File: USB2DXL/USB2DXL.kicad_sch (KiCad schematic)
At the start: 13 parts, among them J1 Conn_01x02, J2 USB_C_Receptacle_USB2.0_16P, U1 CH340E

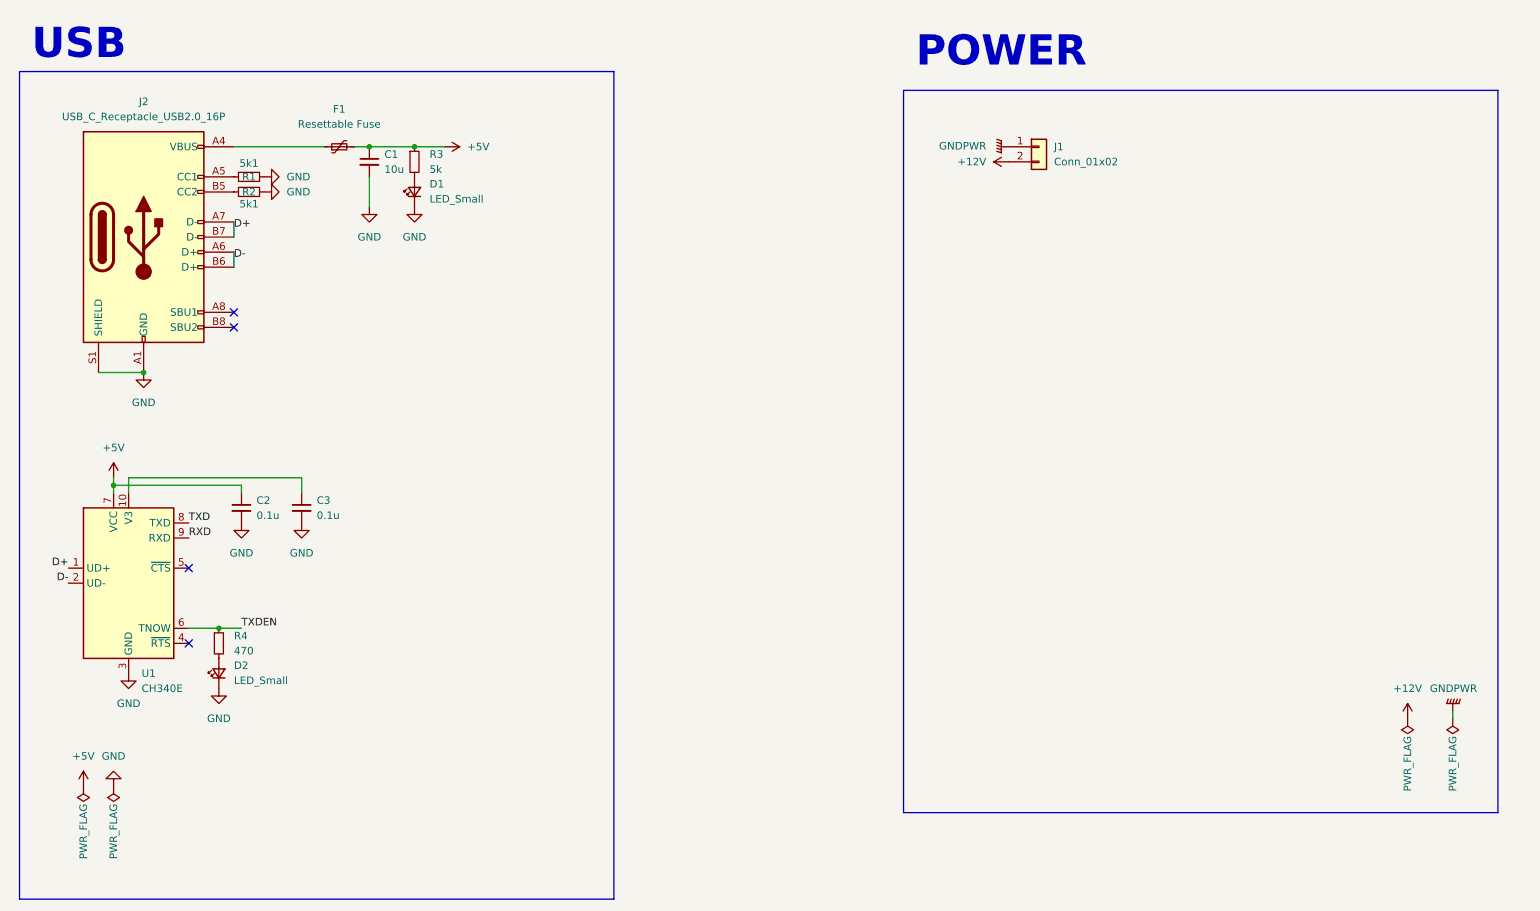
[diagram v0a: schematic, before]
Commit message: 仮
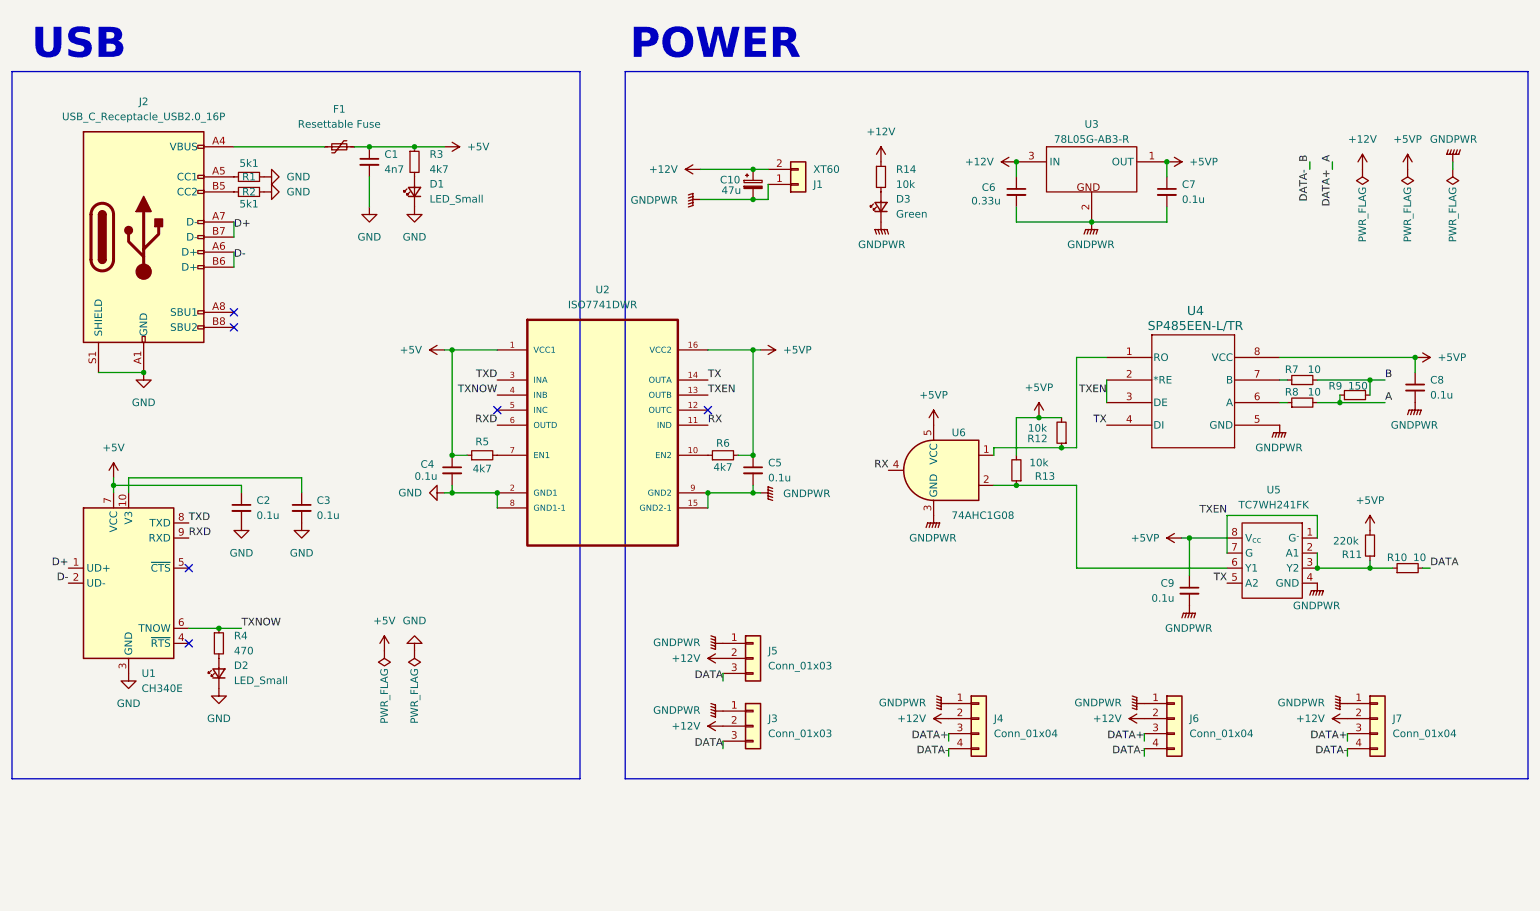
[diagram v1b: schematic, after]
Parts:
- added C10: 47u, Capacitor_THT:CP_Radial_D5.0mm_P2.00mm, symbol Device:C_Polarized_Small
- added C4, C5, C7, C8, C9: 0.1u, Capacitor_SMD:C_0402_1005Metric, symbol Device:C_Small
- added C6: 0.33u, Capacitor_SMD:C_0603_1608Metric, symbol Device:C_Small
- added D3: Green, LED_SMD:LED_0805_2012Metric_Pad1.15x1.40mm_HandSolder, symbol Device:LED_Small
- added J3, J5: Conn_01x03, Connector_JST:JST_EH_B3B-EH-A_1x03_P2.50mm_Vertical, symbol Connector_Generic:Conn_01x03
- added J4, J6, J7: Conn_01x04, Connector_Molex:Molex_SPOX_5267-04A_1x04_P2.50mm_Vertical, symbol Connector_Generic:Conn_01x04
- added R10, R7, R8: 10, Resistor_SMD:R_0402_1005Metric, symbol Device:R_Small
- added R11: 220k, Resistor_SMD:R_0402_1005Metric, symbol Device:R_Small
- added R12, R14: 10k, Resistor_SMD:R_0402_1005Metric, symbol Device:R_Small
- added R13: 10k, Capacitor_SMD:C_0402_1005Metric, symbol Device:R_Small
- added R5, R6: 4k7, Resistor_SMD:R_0402_1005Metric, symbol Device:R_Small
- added R9: 150, Resistor_SMD:R_0402_1005Metric, symbol Device:R_Small
- added U2: ISO7741DWR, ISO7741DWR:SOIC127P1030X265-16N, symbol ISO7741DWR:ISO7741DWR
- added U3: 78L05G-AB3-R, Package_TO_SOT_SMD:SOT-89-3, symbol ProLib_pcs_2025-07-07:78L05G-AB3-R
- added U4: SP485EEN-L/TR, SP485EEN-L/TR:NSOIC-8, symbol SP485EEN-L/TR:SP485EEN-L_TR
- added U5: TC7WH241FK, Package_SO:MSOP-8_3x3mm_P0.65mm, symbol MyLibrary:TC7WH241FK
- added U6: 74AHC1G08, Package_TO_SOT_SMD:SOT-23-5_HandSoldering, symbol 74xGxx:74AHC1G08
- C1: value 10u -> 4n7; footprint (none) -> Capacitor_SMD:C_0402_1005Metric
- C2, C3: footprint (none) -> Capacitor_SMD:C_0402_1005Metric
- D1, D2: footprint (none) -> LED_SMD:LED_0603_1608Metric
- J1: value Conn_01x02 -> XT60
- R1, R2, R4: footprint (none) -> Resistor_SMD:R_0402_1005Metric
- R3: value 5k -> 4k7; footprint (none) -> Resistor_SMD:R_0402_1005Metric
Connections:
- net +12V: now also C10.1, C6.1, J3.2 (Pin_2), J4.2 (Pin_2), J5.2 (Pin_2), J6.2 (Pin_2), J7.2 (Pin_2), R14.1, U3.3 (IN)
- net +5V: now also C4.1, R5.1, U2.1 (VCC1)
- net GND: now also C4.2, U2.2 (GND1), U2.8 (GND1-1)
- net GNDPWR: now also C10.2, C5.2, C6.2, C7.2, C8.2, C9.2, D3.1 (K), J3.1 (Pin_1), J4.1 (Pin_1), J5.1 (Pin_1), J6.1 (Pin_1), J7.1 (Pin_1), U2.15 (GND2-1), U2.9 (GND2), U3.2 (GND), U4.5 (GND), U5.4 (GND), U6.3 (GND)
- net RXD: now also U2.6 (OUTD)
- net TXD: now also U2.3 (INA)
- net TXDEN renamed TXNOW
- net TXNOW: now also U2.4 (INB)
- new net: R13.1, U5.6 (Y1), U6.2
- new net: R12.1, U4.1 (RO), U6.1
- new net: R8.1, U4.6 (A)
- new net: R7.1, U4.7 (B)
- new net: R10.1, R11.1, U5.2 (A1), U5.3 (Y2)
- new net: R5.2, U2.7 (EN1)
- new net: D3.2 (A), R14.2
- new net: R6.1, U2.10 (EN2)
- new net +5VP: C5.1, C7.1, C8.1, C9.1, R11.2, R12.2, R13.2, R6.2, U2.16 (VCC2), U3.1 (OUT), U4.8 (VCC), U5.8 (V_{cc}), U6.5 (VCC)
- new net A: J4.3 (Pin_3), J6.3 (Pin_3), J7.3 (Pin_3), R8.2, R9.1
- new net B: J4.4 (Pin_4), J6.4 (Pin_4), J7.4 (Pin_4), R7.2, R9.2
- new net DATA: J3.3 (Pin_3), J5.3 (Pin_3), R10.2
- new net RX: U2.11 (IND), U6.4
- new net TX: U2.14 (OUTA), U4.4 (DI), U5.5 (A2)
- new net TXEN: U2.13 (OUTB), U4.2 (*RE), U4.3 (DE), U5.1 (G^{-}), U5.7 (G)
- no-connect marks 4 -> 6
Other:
- moved on the sheet: J1
